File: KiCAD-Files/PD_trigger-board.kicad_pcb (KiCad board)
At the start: 2 copper layers, 24 parts, among them J1 USB_C_Receptacle_USB2.0_14P, J10 15V, J11 18V, J2 Conn_01x03, J3 Conn_01x03, J4 VOUT, J5 5V, J6 5V, J7 5V, J8 9V, J9 12V, U1 HUSB238

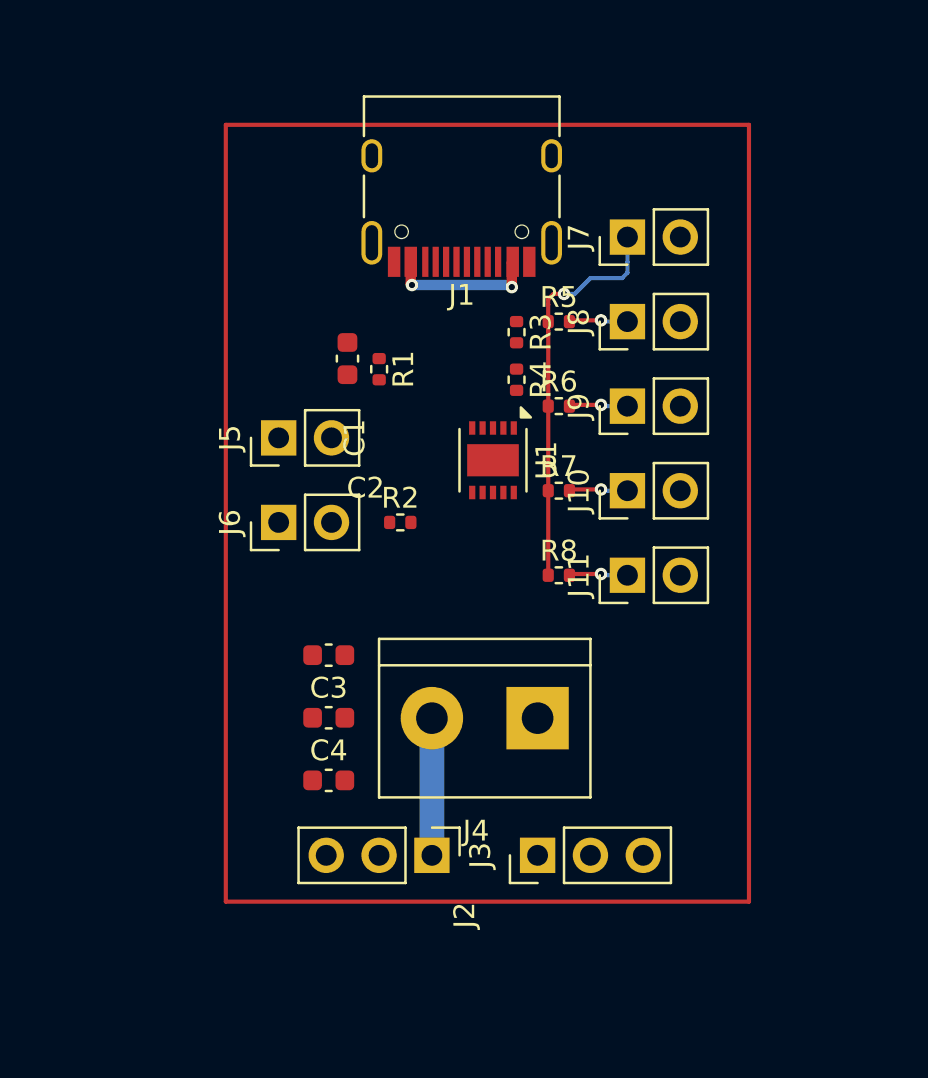
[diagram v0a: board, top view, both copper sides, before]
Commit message: Routin fertig
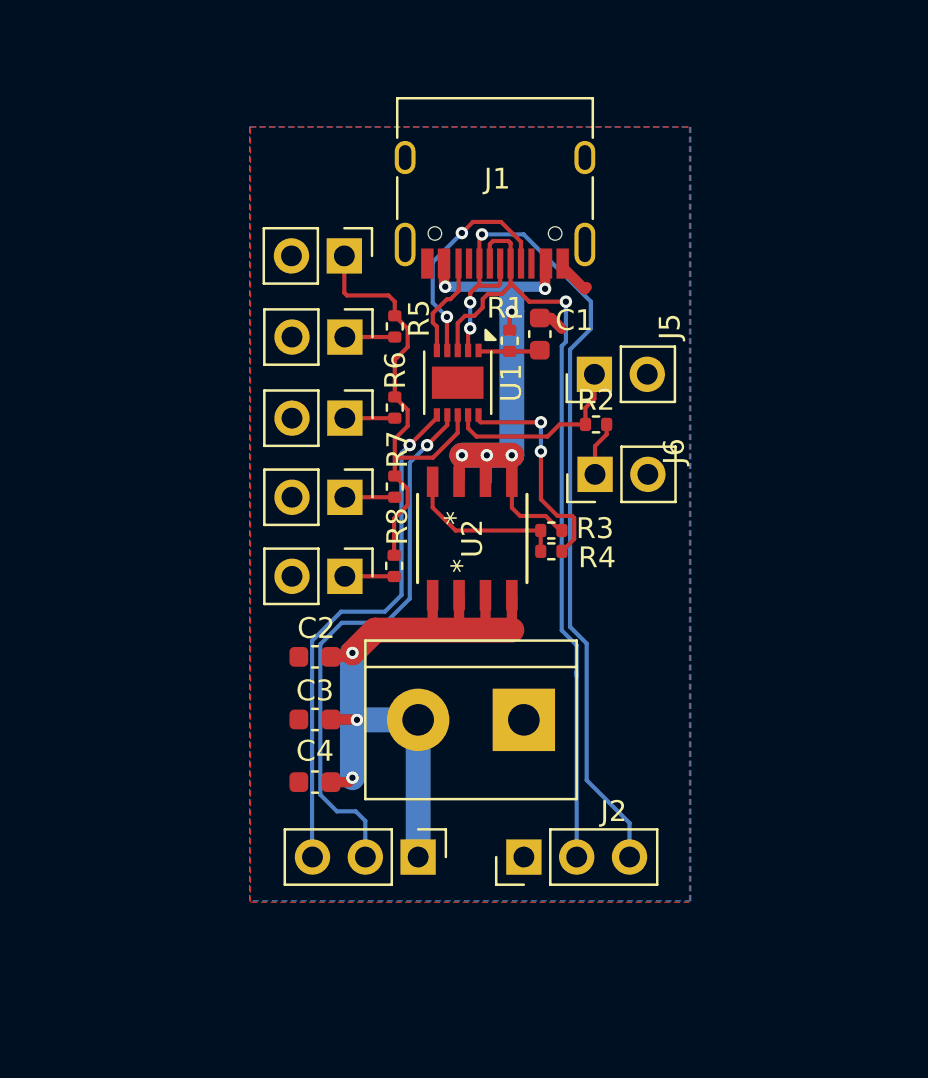
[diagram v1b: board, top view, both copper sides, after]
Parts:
- added U2: SI4459ADY-T1-GE3, blinkyparts:SO_ADY-T1-GE3_VIS, F.Cu at (139.1, 96.1)
- moved J5 15.5 mm to (145.0, 88.2)
- moved J6 15.4 mm to (145.0, 93.0)
- moved J7 13.6 mm to (132.9, 82.5), turned to -90 degrees
- moved J8 13.6 mm to (133.0, 86.4), turned to -90 degrees
- moved J9 13.6 mm to (133.0, 90.3), turned to -90 degrees
- moved J10 13.6 mm to (133.0, 94.1), turned to -90 degrees
- moved J11 13.6 mm to (133.0, 97.9), turned to -90 degrees
- moved R2 10.5 mm to (145.1, 90.6)
- moved R3 9.68 mm to (142.9, 95.7), turned to 180 degrees
- moved C1 9.32 mm to (142.3, 86.3)
- moved R4 8.42 mm to (142.9, 96.7), turned to 0 degrees
- moved R8 7.93 mm to (135.3, 97.4), turned to -90 degrees
- moved R7 7.89 mm to (135.4, 93.6), turned to -90 degrees
- moved R5 7.89 mm to (135.4, 85.9), turned to -90 degrees
- moved R6 7.89 mm to (135.4, 89.8), turned to -90 degrees
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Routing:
- net D+: track 0.00 -> 42.7 mm, vias 0 -> 3
- net D-: track 0.00 -> 39.3 mm, vias 0 -> 1
- net VOUT: track 6.59 -> 33.8 mm, vias 0 -> 3
- net SCL: track 0.00 -> 26.4 mm, vias 0 -> 1
- net SDA: track 0.00 -> 25.0 mm, vias 0 -> 1
- net VBUS: track 7.21 -> 28.7 mm, vias 2 -> 6
- net CC1: track 0.00 -> 11.0 mm, vias 0 -> 2
- net GATE: track 0.00 -> 10.8 mm, vias 0 -> 2
- net ISET: track 0.00 -> 9.27 mm
- net Net-(U2-G): track 0.00 -> 7.92 mm
- net CC2: track 0.00 -> 4.87 mm
- net VSET: track 19.3 -> 22.6 mm, vias 1 -> 0
- net Net-(U1-VIN): track 0.00 -> 3.08 mm
- net GND: track 0.00 -> 3.08 mm
- net Net-(J6-Pin_1): track 0.00 -> 2.63 mm
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- added copper zone on B.Cu, net GND
- added copper zone on F.Cu, net GND
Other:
- board text added: "J5: 1.25A J6 + R2: 4,53 - 1,50A 7,5k - 1,75A 10,5k - 2,00A 13,7k - 2,25A 16,5k - 2,50A 19,6k - 2,75A 22,6k - 3,00A open - 3,25A"
- board text added: "J7: 5V J8: 9V J9: 12V J10: 15V J11: 18V"

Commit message: changed some routing
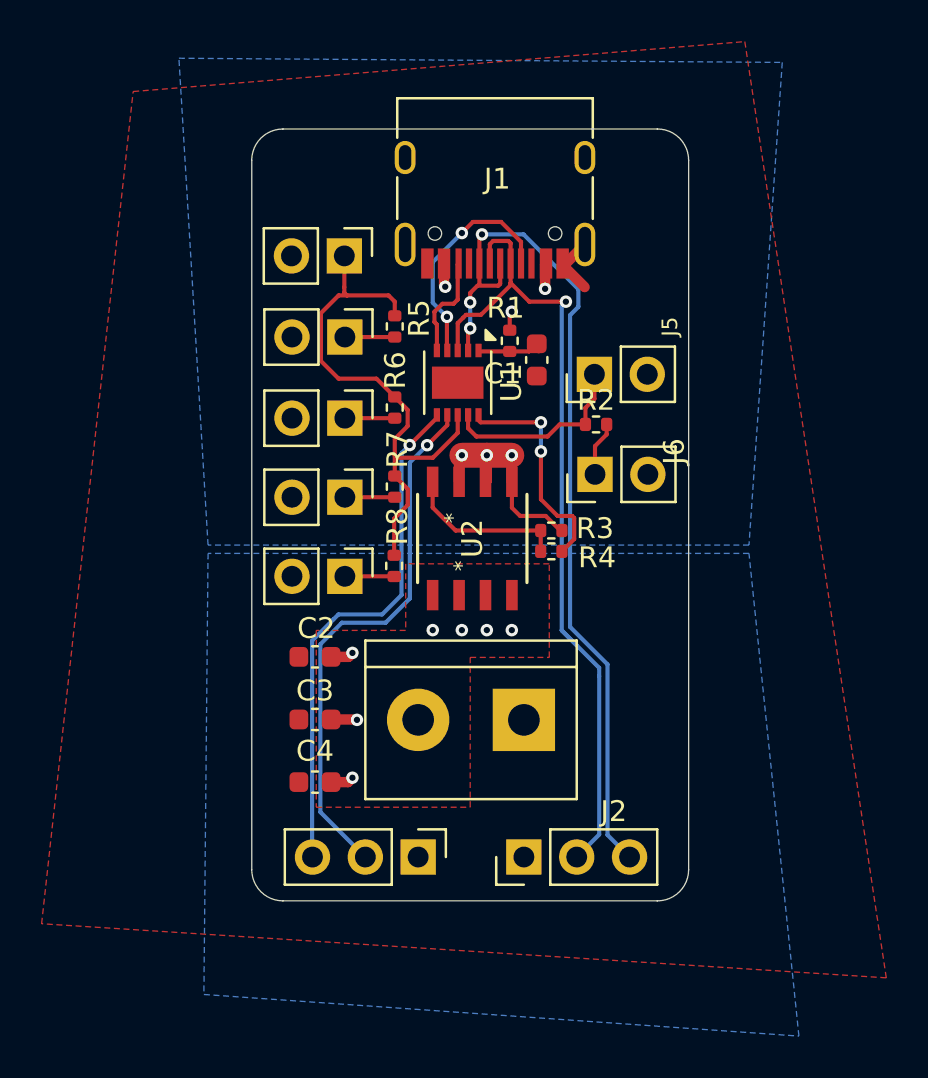
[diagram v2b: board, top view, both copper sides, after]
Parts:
- moved C1 1.25 mm to (142.2, 87.5), turned to -90 degrees
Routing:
- net VOUT: track 33.8 -> 3.50 mm, vias 3 -> 7
- net VBUS: track 28.7 -> 13.7 mm
- net VSET: track 22.6 -> 26.3 mm
- net D-: track 39.3 -> 40.7 mm
- net SCL: track 26.4 -> 25.9 mm
- added copper zone on B.Cu, net VBUS
- added copper zone on B.Cu, net VOUT
- added copper zone on F.Cu, net VOUT
- removed copper zone on B.Cu, net GND
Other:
- board outline added: 21 x 37.1 mm

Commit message: Silkscreen fertig
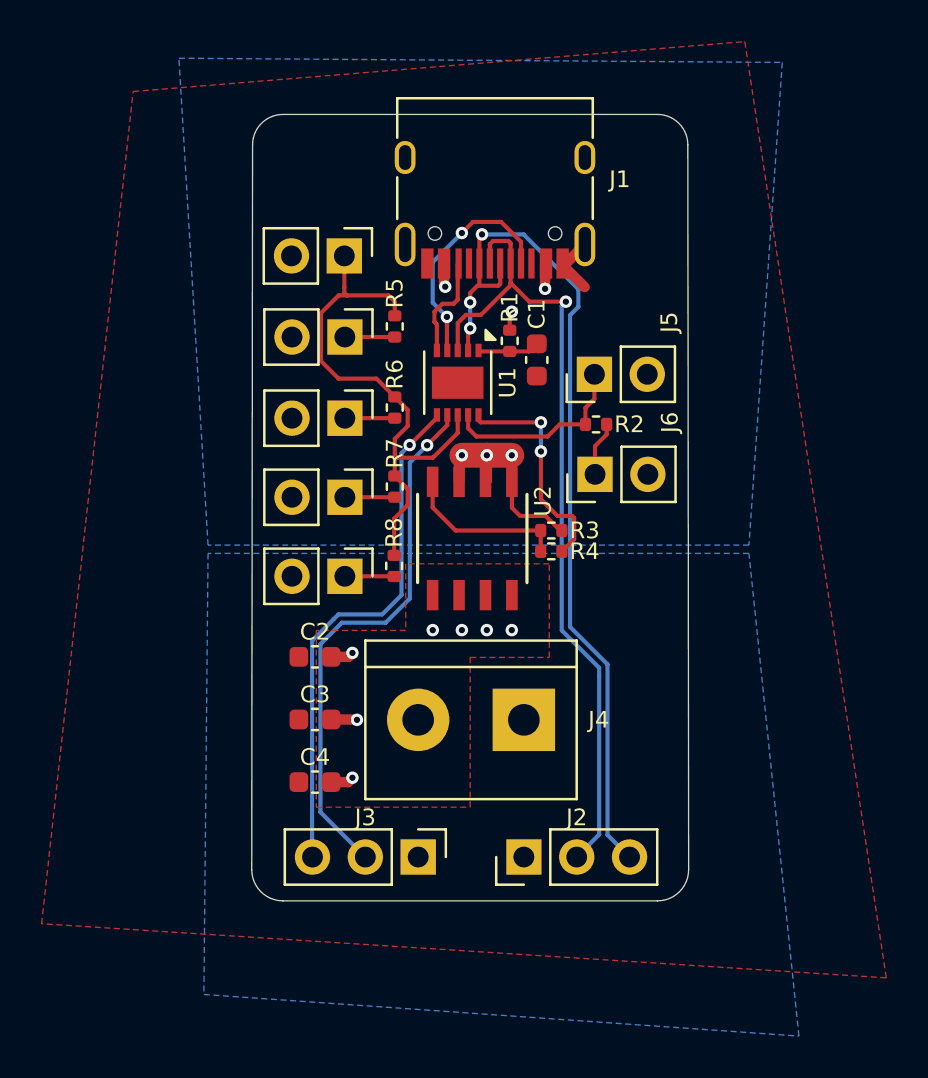
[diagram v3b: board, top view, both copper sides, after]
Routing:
- net D-: track 40.7 -> 39.7 mm
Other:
- board size 21 x 37.1 mm -> 21 x 37.8 mm
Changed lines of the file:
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@@
 		(tags "resistor")
 		(property "Reference" "R5"
-			(at -0.39 -1.17 90)
+			(at -1.6 0 90)
 			(layer "F.SilkS")
 			(effects
 				(font
-					(size 1 1)
-					(thickness 0.15)
+					(size 0.8 0.8)
+					(thickness 0.1)
 				)
 			)
@@
 		(tags "resistor")
 		(property "Reference" "R7"
-			(at -1.79 -0.125 90)
+			(at -1.6 0 90)
 			(layer "F.SilkS")
 			(effects
 				(font
-					(size 1 1)
-					(thickness 0.15)
+					(size 0.8 0.8)
+					(thickness 0.1)
 				)
 			)
@@
 		(tags "usb usb-c 2.0 pd")
 		(property "Reference" "J1"
-			(at -0.107 0.022 0)
+			(at -6 0 0)
 			(layer "F.SilkS")
 			(effects
 				(font
-					(size 1 1)
-					(thickness 0.15)
+					(size 0.8 0.8)
+					(thickness 0.1)
 				)
 			)
@@
 		(tags "resistor")
 		(property "Reference" "R6"
-			(at -1.79 -0.025 90)
+			(at -1.6 0 90)
 			(layer "F.SilkS")
 			(effects
 				(font
-					(size 1 1)
-					(thickness 0.15)
+					(size 0.8 0.8)
+					(thickness 0.1)
 				)
 			)
@@
 		(tags "resistor")
 		(property "Reference" "R3"
-			(at -2.1 0.1 0)
+			(at -1.6 0 0)
 			(layer "F.SilkS")
 			(effects
 				(font
-					(size 1 1)
-					(thickness 0.15)
+					(size 0.8 0.8)
+					(thickness 0.1)
 				)
 			)
@@
 		(tags "Through hole pin header THT 1x03 2.54mm single row")
 		(property "Reference" "J2"
-			(at 2.194 4.32 180)
+			(at 1.9 2.54 180)
 			(layer "F.SilkS")
 			(effects
 				(font
-					(size 1 1)
-					(thickness 0.15)
+					(size 0.8 0.8)
+					(thickness 0.1)
 				)
 			)
@@
 		(tags "resistor")
 		(property "Reference" "R1"
-			(at -1.582 0.2 180)
+			(at -1.6 0 90)
 			(layer "F.SilkS")
 			(effects
 				(font
-					(size 1 1)
-					(thickness 0.15)
+					(size 0.8 0.8)
+					(thickness 0.1)
 				)
 			)
@@
 			(effects
 				(font
-					(size 1 1)
-					(thickness 0.15)
+					(size 0.8 0.8)
+					(thickness 0.1)
 				)
 			)
@@
 			(effects
 				(font
-					(size 1 1)
-					(thickness 0.15)
+					(size 0.8 0.8)
+					(thickness 0.1)
 				)
 			)
@@
 			(effects
 				(font
-					(size 1 1)
-					(thickness 0.15)
+					(size 0.8 0.8)
+					(thickness 0.1)
 				)
 			)
@@
 		(tags "resistor")
 		(property "Reference" "R2"
-			(at 0 -1.17 0)
+			(at 1.6 0 0)
 			(layer "F.SilkS")
 			(effects
 				(font
-					(size 1 1)
-					(thickness 0.15)
+					(size 0.8 0.8)
+					(thickness 0.1)
 				)
 			)
@@
 		(tags "SI4459ADY-T1-GE3 ")
 		(property "Reference" "U2"
-			(at 0 0 90)
+			(at -1.8 -3.4 90)
 			(unlocked yes)
 			(layer "F.SilkS")
 			(effects
 				(font
-					(size 1 1)
-					(thickness 0.15)
+					(size 0.8 0.8)
+					(thickness 0.1)
 				)
 			)
@@
 			(layer "F.Fab")
 		)
-		(fp_text user "*"
-			(at -0.982 1.3 -90)
-			(unlocked yes)
-			(layer "F.SilkS")
-			(effects
-				(font
-					(size 0.75 0.75)
-					(thickness 0.1)
-				)
-			)
-		)
-		(fp_text user "*"
-			(at 1.318 0.5 90)
-			(unlocked yes)
-			(layer "F.SilkS")
-			(effects
-				(font
-					(size 0.75 0.75)
-					(thickness 0.1)
-				)
-			)
-		)
 		(fp_text user "${REFERENCE}"
 			(at 0 0 -90)
@@
 		(tags "terminal block bornier2")
 		(property "Reference" "J4"
-			(at -3.62 -0.4 0)
-			(layer "B.SilkS")
+			(at -3.6 0 0)
+			(layer "F.SilkS")
 			(effects
 				(font
-					(size 1 1)
+					(size 0.8 0.8)
 					(thickness 0.15)
 				)
@@
 		(tags "capacitor")
 		(property "Reference" "C2"
-			(at -0.06 1.372 0)
+			(at 0 1.2 0)
 			(layer "F.SilkS")
 			(effects
 				(font
-					(size 1 1)
-					(thickness 0.15)
+					(size 0.8 0.8)
+					(thickness 0.1)
 				)
 			)
@@
 		(tags "resistor")
 		(property "Reference" "R8"
-			(at -1.9 -0.155 90)
+			(at -1.6 0 90)
 			(layer "F.SilkS")
 			(effects
 				(font
-					(size 1 1)
-					(thickness 0.15)
+					(size 0.8 0.8)
+					(thickness 0.1)
 				)
 			)
@@
 		(tags "Through hole pin header THT 1x02 2.54mm single row")
 		(property "Reference" "J5"
-			(at 2.29 3.629 90)
+			(at 2.5 3.6 90)
 			(layer "F.SilkS")
 			(effects
 				(font
-					(size 0.75 0.75)
+					(size 0.8 0.8)
 					(thickness 0.1)
 				)
@@
 		(tags "Through hole pin header THT 1x02 2.54mm single row")
 		(property "Reference" "J8"
-			(at 0 3.85 -90)
+			(at 0 3.85 270)
 			(layer "B.SilkS")
 			(effects
 				(font
-					(size 1 1)
-					(thickness 0.15)
+					(size 0.8 0.8)
+					(thickness 0.1)
 				)
 			)
@@
 		(tags "DFN 0.5")
 		(property "Reference" "U1"
-			(at 0 -2.575 90)
+			(at 0 -2.4 90)
 			(layer "F.SilkS")
 			(effects
 				(font
-					(size 1 1)
-					(thickness 0.15)
+					(size 0.8 0.8)
+					(thickness 0.1)
 				)
 			)
@@
 		(tags "resistor")
 		(property "Reference" "R4"
-			(at 2.2 0.3 0)
+			(at 1.6 0 0)
 			(layer "F.SilkS")
 			(effects
 				(font
-					(size 1 1)
-					(thickness 0.15)
+					(size 0.8 0.8)
+					(thickness 0.1)
 				)
 			)
@@
 		(tags "capacitor")
 		(property "Reference" "C4"
-			(at 0 1.492 0)
+			(at 0 1.2 0)
 			(layer "F.SilkS")
 			(effects
 				(font
-					(size 1 1)
-					(thickness 0.15)
+					(size 0.8 0.8)
+					(thickness 0.1)
 				)
 			)
@@
 		(tags "capacitor")
 		(property "Reference" "C3"
-			(at 0 1.382 0)
+			(at 0 1.2 0)
 			(layer "F.SilkS")
 			(effects
 				(font
-					(size 1 1)
-					(thickness 0.15)
+					(size 0.8 0.8)
+					(thickness 0.1)
 				)
 			)
@@
 		(tags "Through hole pin header THT 1x02 2.54mm single row")
 		(property "Reference" "J6"
-			(at 1.1 3.8 90)
+			(at 2.5 3.6 90)
 			(layer "F.SilkS")
 			(effects
 				(font
-					(size 1 1)
-					(thickness 0.15)
+					(size 0.8 0.8)
+					(thickness 0.1)
 				)
 			)
@@
 		(tags "Through hole pin header THT 1x03 2.54mm single row")
 		(property "Reference" "J3"
-			(at -1.894 0.8 180)
-			(layer "B.SilkS")
+			(at -1.9 2.54 180)
+			(layer "F.SilkS")
 			(effects
 				(font
-					(size 1 1)
-					(thickness 0.15)
+					(size 0.8 0.8)
+					(thickness 0.1)
 				)
 			)
@@
 			(effects
 				(font
-					(size 1 1)
-					(thickness 0.15)
+					(size 0.8 0.8)
+					(thickness 0.1)
 				)
 				(justify mirror)
@@
 		(tags "capacitor")
 		(property "Reference" "C1"
-			(at 0.6595 1.6525 360)
+			(at -2.2 0 90)
 			(layer "F.SilkS")
 			(effects
 				(font
-					(size 1 1)
-					(thickness 0.15)
+					(size 0.8 0.8)
+					(thickness 0.1)
 				)
 			)
@@
 	)
 	(gr_line
-		(start 148 76.4)
-		(end 130 76.4)
+		(start 148 75.7)
+		(end 130 75.7)
 		(stroke
 			(width 0.05)
@@
 	(gr_line
 		(start 149.5 112)
-		(end 149.5 77.9)
+		(end 149.46066 77.16066)
 		(stroke
 			(width 0.05)
@@
 	)
 	(gr_line
-		(start 128.5 77.9)
+		(start 128.539566 77.16066)
 		(end 128.5 112)
 		(stroke
@@
 	)
 	(gr_arc
-		(start 148 76.4)
-		(mid 149.06066 76.83934)
-		(end 149.5 77.9)
+		(start 148 75.7)
+		(mid 149.032843 76.127817)
+		(end 149.46066 77.16066)
 		(stroke
 			(width 0.05)
@@
 	)
 	(gr_arc
-		(start 128.5 77.9)
-		(mid 128.93934 76.83934)
-		(end 130 76.4)
+		(start 128.539566 77.16066)
+		(mid 128.967317 76.127977)
+		(end 130 75.700226)
 		(stroke
 			(width 0.05)
@@
 	)
 	(gr_text " J7:  5V\n J8:  9V\n J9: 12V\nJ10: 15V\nJ11: 18V"
-		(at 140.3 89.8 0)
+		(at 139.7 99.1 0)
 		(layer "B.SilkS")
 		(effects
 			(font
-				(size 1 1)
+				(size 0.8 0.8)
 				(thickness 0.1)
 			)
@@
 	)
 	(gr_text "J5:     1.25A\nJ6 + R2:\n 4,53 - 1,50A\n 7,5k - 1,75A\n10,5k - 2,00A\n13,7k - 2,25A\n16,5k - 2,50A\n19,6k - 2,75A\n22,6k - 3,00A\nopen  - 3,25A"
-		(at 148.6 109.5 0)
+		(at 143.6 92.8 0)
 		(layer "B.SilkS")
 		(effects
 			(font
-				(size 0.75 0.75)
+				(size 0.8 0.8)
 				(thickness 0.1)
 			)
@@
 		(width 0.2)
 		(layer "B.Cu")
-		(net 4)
-	)
-	(segment
-		(start 143.4 100.5)
-		(end 144.12 101.22)
-		(width 0.2)
-		(layer "B.Cu")
